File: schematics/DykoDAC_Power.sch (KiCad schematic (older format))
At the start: 40 parts, among them J1 AC Input, U1 LT1762-5, U2 LM317, U3 LM337, U4 L7805, U5 78L05, U6 LP5907-3.3, U7 LP5907-3.3

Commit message: pcb update
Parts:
- U2, U3, U4: footprint TO_SOT_Packages_SMD:SOT-223-3_TabPin2 -> TO_SOT_Packages_SMD:TO-263-2
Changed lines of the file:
@@
 F 0 "U4" H 7150 2342 50  0000 C CNN
 F 1 "L7805" H 7150 2251 50  0000 C CNN
-F 2 "TO_SOT_Packages_SMD:SOT-223-3_TabPin2" H 7175 1950 50  0001 L CIN
+F 2 "TO_SOT_Packages_SMD:TO-263-2" H 7175 1950 50  0001 L CIN
 F 3 "http://www.st.com/content/ccc/resource/technical/document/datasheet/41/4f/b3/b0/12/d4/47/88/CD00000444.pdf/files/CD00000444.pdf/jcr:content/translations/en.CD00000444.pdf" H 7150 2050 50  0001 C CNN
 	1    7150 2100
@@
 F 0 "U3" H 3700 2701 50  0000 C CNN
 F 1 "LM337" H 3700 2610 50  0000 C CNN
-F 2 "TO_SOT_Packages_SMD:SOT-223-3_TabPin2" H 3700 2650 50  0001 C CIN
+F 2 "TO_SOT_Packages_SMD:TO-263-2" H 3700 2650 50  0001 C CIN
 F 3 "http://www.ti.com/lit/ds/symlink/lm337-n.pdf" H 3700 2850 50  0001 C CNN
 	1    3700 2850
@@
 F 0 "U2" H 3700 1208 50  0000 C CNN
 F 1 "LM317" H 3700 1299 50  0000 C CNN
-F 2 "TO_SOT_Packages_SMD:SOT-223-3_TabPin2" H 3700 1250 50  0001 C CIN
+F 2 "TO_SOT_Packages_SMD:TO-263-2" H 3700 1250 50  0001 C CIN
 F 3 "http://www.ti.com/lit/ds/symlink/lm337-n.pdf" H 3700 1450 50  0001 C CNN
 	1    3700 1450

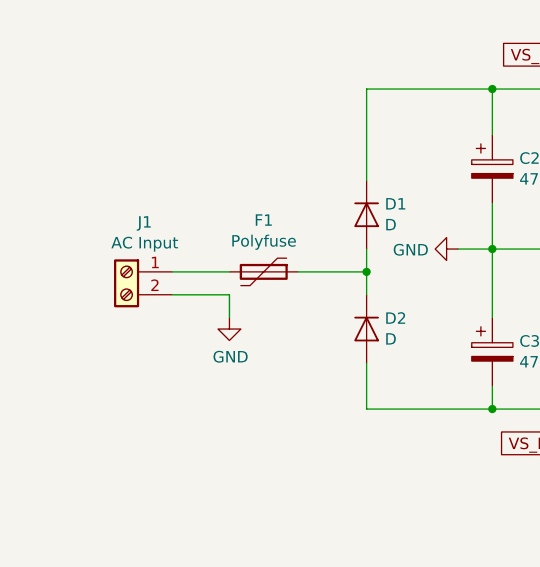
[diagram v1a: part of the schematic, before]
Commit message: switch
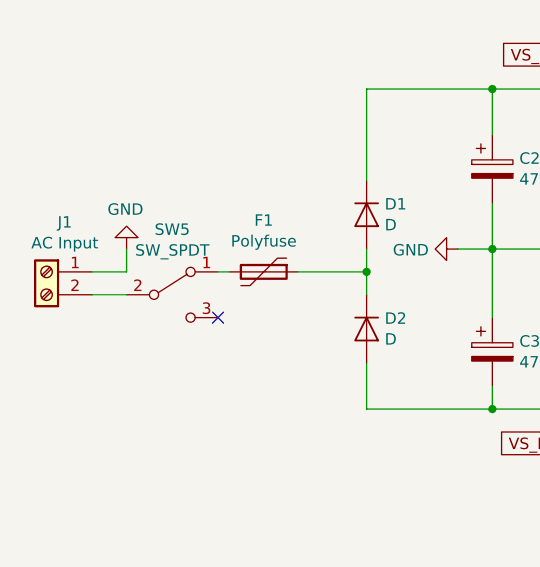
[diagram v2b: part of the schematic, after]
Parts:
- added SW5: SW_SPDT, Button_Switch_THT:SW_Push_1P2T_Vertical_E-Switch_800UDP8P1A1M6, symbol Switch:SW_SPDT
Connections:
- net GND: now also J1.1 (Pin_1); no longer J1.2 (Pin_2)
- net at F1.2: now also SW5.1 (A); no longer J1.1 (Pin_1)
- new net: J1.2 (Pin_2), SW5.2 (B)
- no-connect marks 0 -> 1
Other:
- moved on the sheet: J1
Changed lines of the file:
@@
 L Connector:Screw_Terminal_01x02 J1
 U 1 1 5C8C0A04
-P 1150 2250
-F 0 "J1" H 1070 2467 50  0000 C CNN
-F 1 "AC Input" H 1070 2376 50  0000 C CNN
-F 2 "Terminal_Blocks:TerminalBlock_Altech_AK300-2_P5.00mm" H 1150 2250 50  0001 C CNN
-F 3 "~" H 1150 2250 50  0001 C CNN
-	1    1150 2250
+P 800 2250
+F 0 "J1" H 720 2467 50  0000 C CNN
+F 1 "AC Input" H 720 2376 50  0000 C CNN
+F 2 "Terminal_Blocks:TerminalBlock_Altech_AK300-2_P5.00mm" H 800 2250 50  0001 C CNN
+F 3 "~" H 800 2250 50  0001 C CNN
+	1    800  2250
 	-1   0    0    -1
 $EndComp
@@
 L power:GND #PWR01
 U 1 1 5C8C1266
-P 1600 2450
-F 0 "#PWR01" H 1600 2200 50  0001 C CNN
-F 1 "GND" H 1605 2277 50  0000 C CNN
-F 2 "" H 1600 2450 50  0001 C CNN
-F 3 "" H 1600 2450 50  0001 C CNN
-	1    1600 2450
-	1    0    0    -1
+P 1150 2150
+F 0 "#PWR01" H 1150 1900 50  0001 C CNN
+F 1 "GND" H 1155 1977 50  0000 C CNN
+F 2 "" H 1150 2150 50  0001 C CNN
+F 3 "" H 1150 2150 50  0001 C CNN
+	1    1150 2150
+	-1   0    0    1
 $EndComp
 $Comp
@@
 	2200 2150 2200 2250
 Wire Wire Line
-	1350 2350 1600 2350
-Wire Wire Line
-	1600 2350 1600 2450
-Wire Wire Line
-	1350 2250 1600 2250
+	1150 2250 1150 2150
 Wire Wire Line
 	1900 2250 2200 2250
@@
 	9850 2700 9400 2700
 Connection ~ 9400 2700
+$Comp
+L Switch:SW_SPDT SW5
+U 1 1 5E682A1D
+P 1350 2350
+F 0 "SW5" H 1350 2635 50  0000 C CNN
+F 1 "SW_SPDT" H 1350 2544 50  0000 C CNN
+F 2 "Button_Switch_THT:SW_Push_1P2T_Vertical_E-Switch_800UDP8P1A1M6" H 1350 2350 50  0001 C CNN
+F 3 "~" H 1350 2350 50  0001 C CNN
+	1    1350 2350
+	1    0    0    -1
+$EndComp
+Wire Wire Line
+	1600 2250 1550 2250
+Wire Wire Line
+	1150 2350 1000 2350
+Wire Wire Line
+	1150 2250 1000 2250
+NoConn ~ 1550 2450
 $EndSCHEMATC

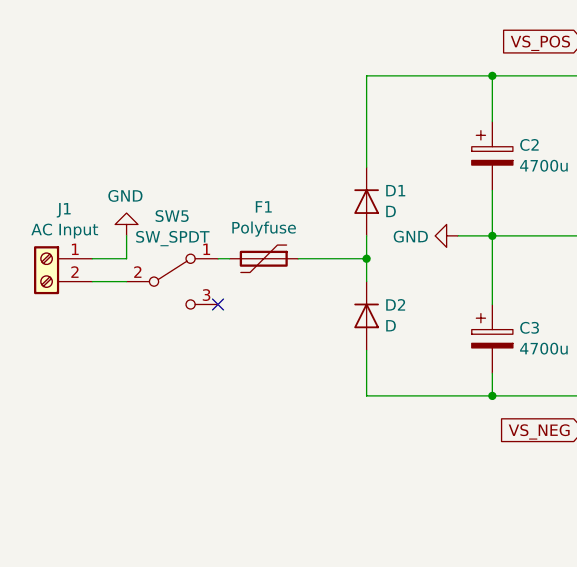
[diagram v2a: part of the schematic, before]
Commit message: update
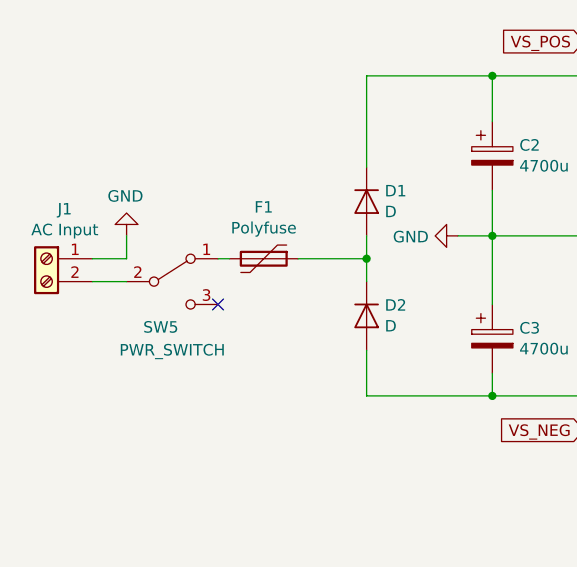
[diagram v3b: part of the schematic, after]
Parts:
- C14, C15, C64, C65, C9: footprint Capacitors_Tantalum_SMD:CP_Tantalum_Case-A_EIA-3216-18_Reflow -> Capacitor_Tantalum_SMD:CP_EIA-3216-18_Kemet-A
- C49, C7, C8: footprint Capacitors_Tantalum_SMD:CP_Tantalum_Case-D_EIA-7343-31_Reflow -> Capacitor_Tantalum_SMD:CP_EIA-7343-31_Kemet-D
- SW5: value SW_SPDT -> PWR_SWITCH
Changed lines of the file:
@@
 F 0 "C8" H 5068 2546 50  0000 L CNN
 F 1 "100u" H 5068 2455 50  0000 L CNN
-F 2 "Capacitors_Tantalum_SMD:CP_Tantalum_Case-D_EIA-7343-31_Reflow" H 4988 2350 50  0001 C CNN
+F 2 "Capacitor_Tantalum_SMD:CP_EIA-7343-31_Kemet-D" H 4988 2350 50  0001 C CNN
 F 3 "~" H 4950 2500 50  0001 C CNN
 	1    4950 2500
@@
 F 0 "C7" H 5068 1846 50  0000 L CNN
 F 1 "100u" H 5068 1755 50  0000 L CNN
-F 2 "Capacitors_Tantalum_SMD:CP_Tantalum_Case-D_EIA-7343-31_Reflow" H 4988 1650 50  0001 C CNN
+F 2 "Capacitor_Tantalum_SMD:CP_EIA-7343-31_Kemet-D" H 4988 1650 50  0001 C CNN
 F 3 "~" H 4950 1800 50  0001 C CNN
 F 4 "TAJD107K016SNJ " H 4950 1800 50  0001 C CNN "Part"
@@
 F 0 "C9" H 4818 4696 50  0000 L CNN
 F 1 "10u" H 4818 4605 50  0000 L CNN
-F 2 "Capacitors_Tantalum_SMD:CP_Tantalum_Case-A_EIA-3216-18_Reflow" H 4738 4500 50  0001 C CNN
+F 2 "Capacitor_Tantalum_SMD:CP_EIA-3216-18_Kemet-A" H 4738 4500 50  0001 C CNN
 F 3 "~" H 4700 4650 50  0001 C CNN
 F 4 "T491A106K016AT " H 4700 4650 50  0001 C CNN "Part"
@@
 F 0 "C14" H 7668 2396 50  0000 L CNN
 F 1 "10u" H 7668 2305 50  0000 L CNN
-F 2 "Capacitors_Tantalum_SMD:CP_Tantalum_Case-A_EIA-3216-18_Reflow" H 7588 2200 50  0001 C CNN
+F 2 "Capacitor_Tantalum_SMD:CP_EIA-3216-18_Kemet-A" H 7588 2200 50  0001 C CNN
 F 3 "~" H 7550 2350 50  0001 C CNN
 	1    7550 2350
@@
 F 0 "C15" H 7550 4750 50  0000 L CNN
 F 1 "10u" H 7350 4550 50  0000 L CNN
-F 2 "Capacitors_Tantalum_SMD:CP_Tantalum_Case-A_EIA-3216-18_Reflow" H 7588 4500 50  0001 C CNN
+F 2 "Capacitor_Tantalum_SMD:CP_EIA-3216-18_Kemet-A" H 7588 4500 50  0001 C CNN
 F 3 "~" H 7550 4650 50  0001 C CNN
 	1    7550 4650
@@
 F 0 "C64" H 3788 1996 50  0000 L CNN
 F 1 "10u" H 3800 1900 50  0000 L CNN
-F 2 "Capacitors_Tantalum_SMD:CP_Tantalum_Case-A_EIA-3216-18_Reflow" H 3700 1950 50  0001 C CNN
+F 2 "Capacitor_Tantalum_SMD:CP_EIA-3216-18_Kemet-A" H 3700 1950 50  0001 C CNN
 F 3 "~" H 3700 1950 50  0001 C CNN
 	1    3700 1950
@@
 F 0 "C65" H 3788 2396 50  0000 L CNN
 F 1 "10u" H 3800 2300 50  0000 L CNN
-F 2 "Capacitors_Tantalum_SMD:CP_Tantalum_Case-A_EIA-3216-18_Reflow" H 3700 2350 50  0001 C CNN
+F 2 "Capacitor_Tantalum_SMD:CP_EIA-3216-18_Kemet-A" H 3700 2350 50  0001 C CNN
 F 3 "~" H 3700 2350 50  0001 C CNN
 	1    3700 2350
@@
 F 0 "C49" H 9968 2396 50  0000 L CNN
 F 1 "100u" H 9968 2305 50  0000 L CNN
-F 2 "Capacitors_Tantalum_SMD:CP_Tantalum_Case-D_EIA-7343-31_Reflow" H 9888 2200 50  0001 C CNN
+F 2 "Capacitor_Tantalum_SMD:CP_EIA-7343-31_Kemet-D" H 9888 2200 50  0001 C CNN
 F 3 "~" H 9850 2350 50  0001 C CNN
 	1    9850 2350
@@
 U 1 1 5E682A1D
 P 1350 2350
-F 0 "SW5" H 1350 2635 50  0000 C CNN
-F 1 "SW_SPDT" H 1350 2544 50  0000 C CNN
+F 0 "SW5" H 1300 2150 50  0000 C CNN
+F 1 "PWR_SWITCH" H 1350 2050 50  0000 C CNN
 F 2 "Button_Switch_THT:SW_Push_1P2T_Vertical_E-Switch_800UDP8P1A1M6" H 1350 2350 50  0001 C CNN
 F 3 "~" H 1350 2350 50  0001 C CNN
